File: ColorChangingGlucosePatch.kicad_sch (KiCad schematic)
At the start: 6 parts, among them U1 TPS76925DBVR, U2 TPS76925DBVR

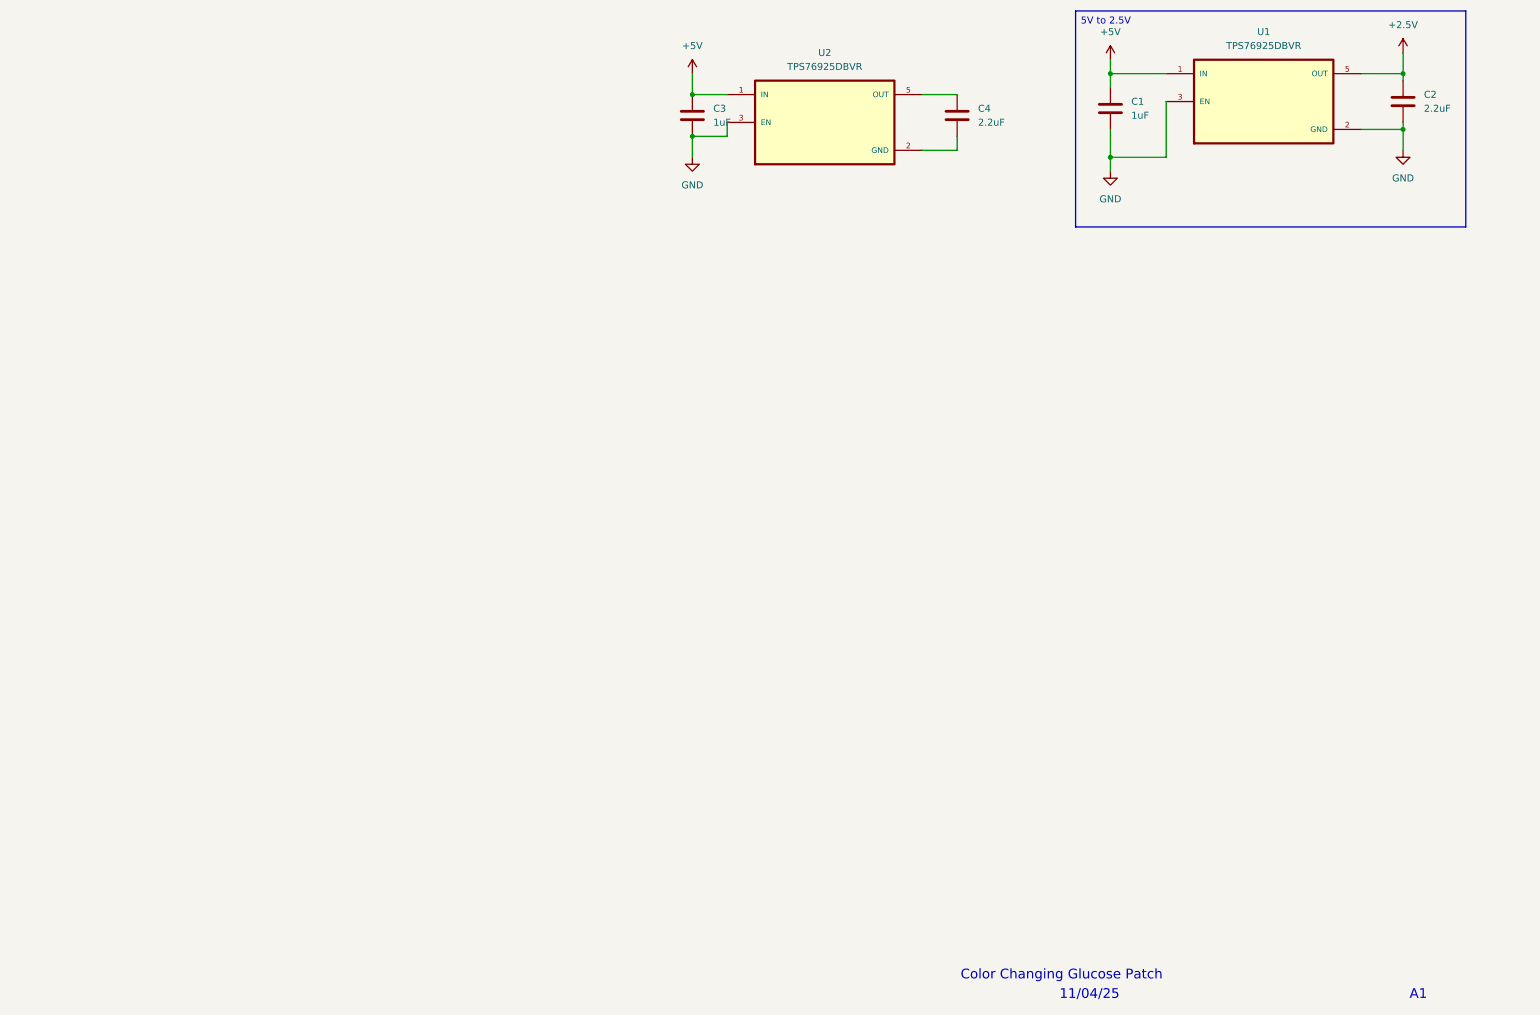
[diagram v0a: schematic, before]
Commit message: holy shit its working
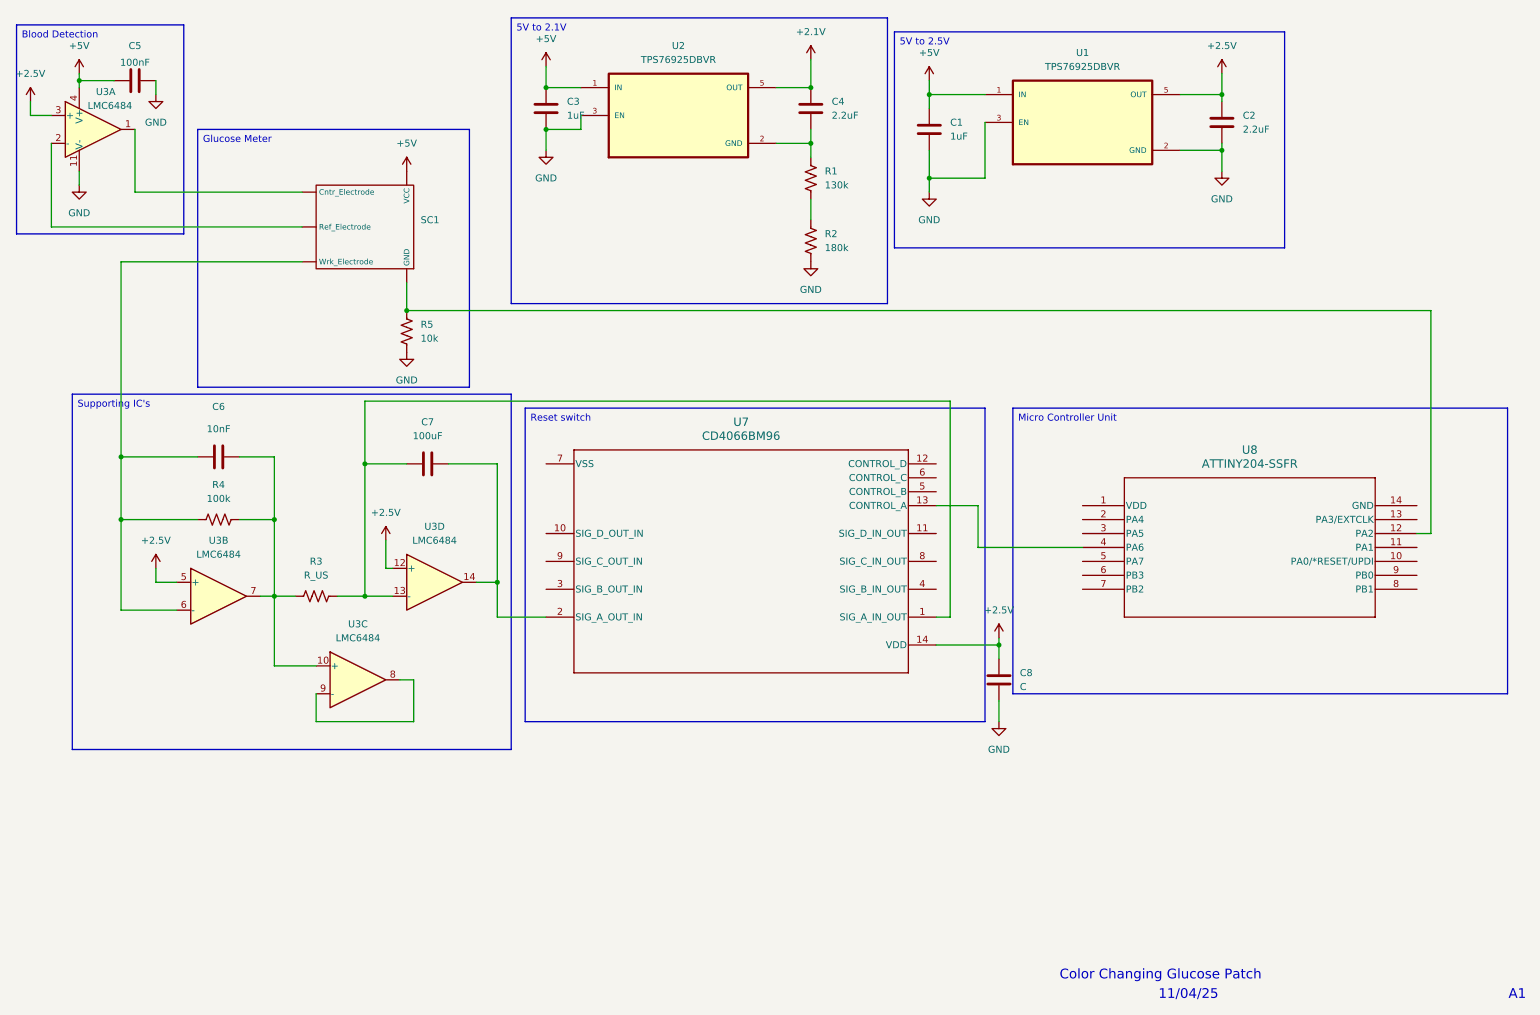
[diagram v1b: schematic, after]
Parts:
- added C5: 100nF, Capacitor_SMD:CP_Elec_3x5.3, symbol Device:C
- added C6: 10nF, Capacitor_SMD:CP_Elec_3x5.3, symbol Device:C
- added C7: 100uF, Capacitor_SMD:CP_Elec_3x5.3, symbol Device:C
- added C8: C, Capacitor_SMD:CP_Elec_3x5.3, symbol Device:C
- added R1: 130k, Resistor_SMD:R_0201_0603Metric, symbol Device:R_US
- added R2: 180k, Resistor_SMD:R_0201_0603Metric, symbol Device:R_US
- added R3: R_US, Resistor_SMD:R_0201_0603Metric_Pad0.64x0.40mm_HandSolder, symbol Device:R_US
- added R4: 100k, Resistor_SMD:R_0201_0603Metric_Pad0.64x0.40mm_HandSolder, symbol Device:R_US
- added R5: 10k, Resistor_SMD:R_0201_0603Metric_Pad0.64x0.40mm_HandSolder, symbol Device:R_US
- added SC1: ~, Glucose Meter:Strip-Connector, symbol Glucose_meter:Strip_Connector
- added U3: LMC6484, LMC6484AIN_NOPB-2:DIP254P762X508-14, symbol Amplifier_Operational:LMC6484
- added U7: CD4066BM96, footprints:D0014A_N, symbol CD4066:CD4066BM96
- added U8: ATTINY204-SSFR, ATTINY204_SSFR:SOIC14_SL_MCH, symbol ATTINY204_SSFR:ATTINY204-SSFR
- C1, C2, C3, C4: footprint (none) -> Capacitor_SMD:CP_Elec_3x5.3
- U1, U2: footprint TPS76925DBVR:SOT95P280X145-5N -> TPS76925DBVR-2:SOT95P280X145-5N
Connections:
- net +2.5V: now also C8.1, U3.12 (+), U3.3 (+), U3.5 (+), U7.14 (VDD)
- net +5V: now also C5.1, SC1. (Cntr_Electrode), U3.4 (V+)
- net GND: now also C5.2, C8.2, R2.2, R5.2, U3.11 (V-)
- net at C4.2, U2.2 (GND): now also R1.1
- net +2.1V: now reaches C4.1, U2.5 (OUT)
- new net: C7.1, R3.2, U3.13 (-), U7.1 (SIG_A_IN_OUT)
- new net: C7.2, U3.14, U7.2 (SIG_A_OUT_IN)
- new net: SC1. (Cntr_Electrode), U3.1
- new net: SC1. (Cntr_Electrode), U3.2 (-)
- new net: C6.2, R3.1, R4.2, U3.10 (+), U3.7
- new net: U3.8, U3.9 (-)
- new net: C6.1, R4.1, SC1. (Cntr_Electrode), U3.6 (-)
- new net: R5.1, SC1. (Cntr_Electrode), U8.12 (PA2)
- new net: U7.13 (CONTROL_A), U8.4 (PA6)
- new net: R1.2, R2.1
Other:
- moved on the sheet: C1, C2, C3, C4, U1, U2
